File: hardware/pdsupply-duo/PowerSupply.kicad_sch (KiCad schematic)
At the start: 8 parts, among them U5 LTM8026IV#PBF, U6 ACS71240KEXBLT-050U5

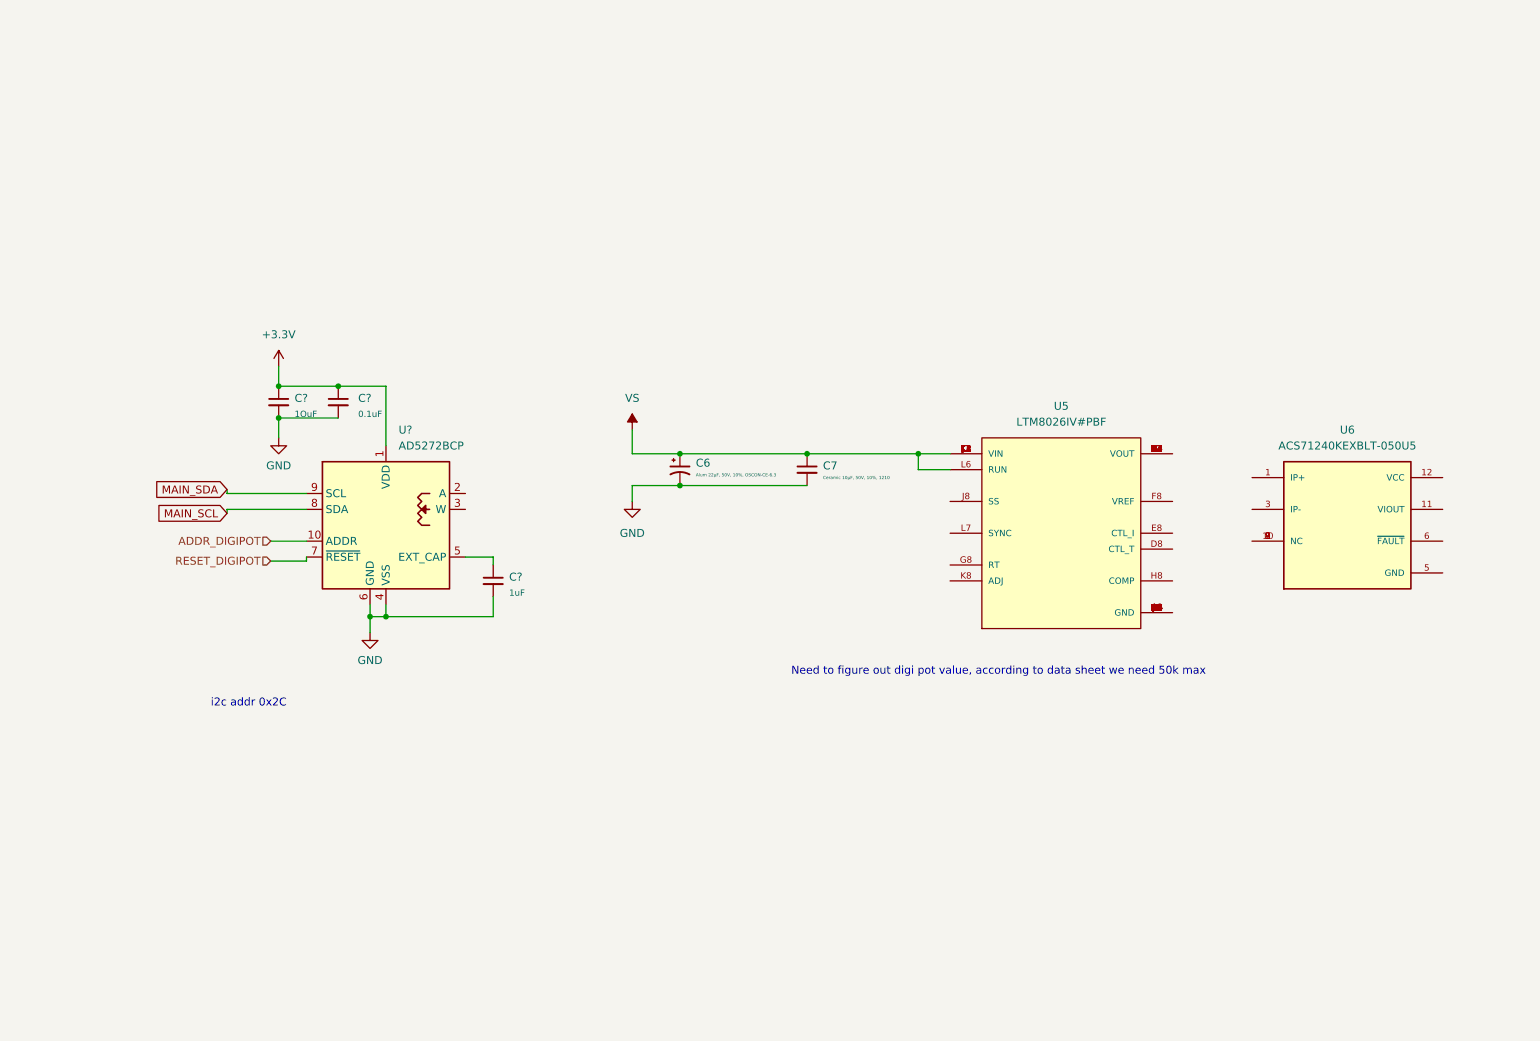
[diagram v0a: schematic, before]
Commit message: SCH 85% done
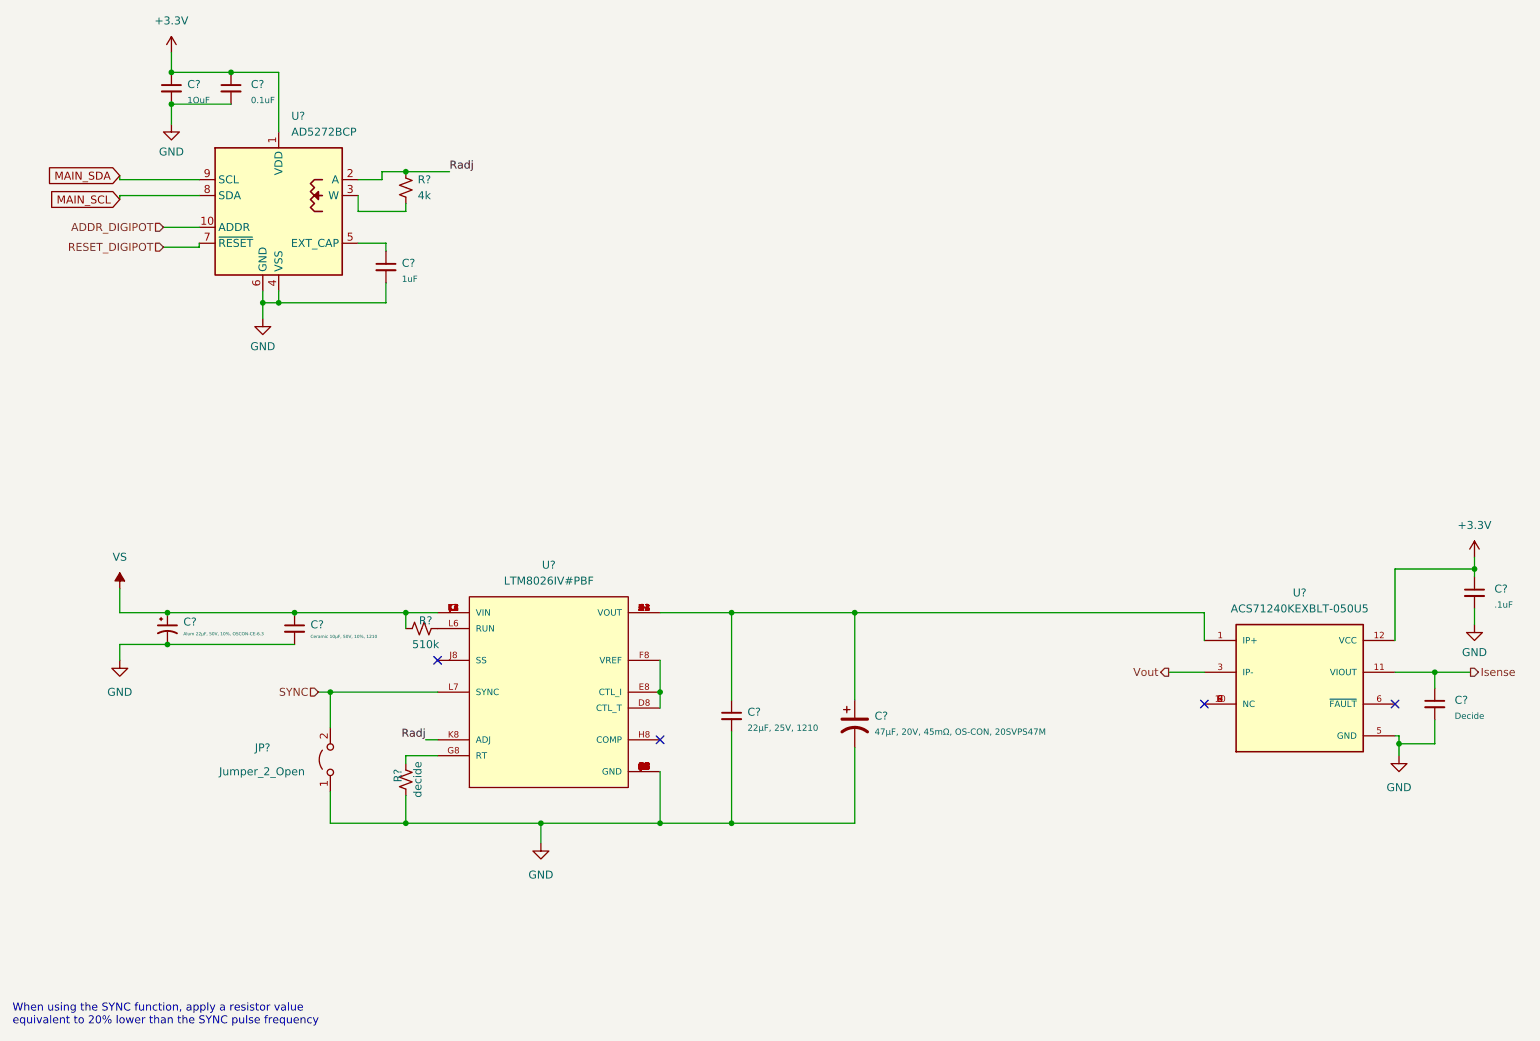
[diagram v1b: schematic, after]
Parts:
- added C?: .1uF, symbol Device:C_Small
- added C?: 22µF, 25V, 1210, symbol Device:C_Small
- added C?: Decide, symbol Device:C_Small
- added C?: 47µF, 20V, 45mΩ, OS-CON, 20SVPS47M, symbol Device:C_Polarized_US
- added JP?: Jumper_2_Open, symbol Jumper:Jumper_2_Open
- added R?: 4k, symbol Device:R_Small_US
- added R?: decide, symbol Device:R_Small_US
- added R?: 510k, symbol Device:R_Small_US
- renumbered C7 to C?, C6 to C?, U6 to U?, U5 to U?
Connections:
- net +3V3: now also U?.12 (VCC), C?.1
- net GND: now also U?.5 (GND), U?.A5 (GND), U?.A6 (GND), U?.A7 (GND), U?.A8 (GND), U?.B5 (GND), U?.B6 (GND), U?.B7 (GND), U?.B8 (GND), U?.C5 (GND), U?.C6 (GND), U?.C7 (GND), U?.C8 (GND), U?.D5 (GND), U?.D6 (GND), U?.D7 (GND), U?.E1 (GND), U?.E2 (GND), U?.E3 (GND), U?.E4 (GND), U?.E5 (GND), U?.E6 (GND), U?.E7 (GND), U?.F1 (GND), U?.F2 (GND), U?.F3 (GND), U?.F4 (GND), U?.F5 (GND), U?.F6 (GND), U?.F7 (GND), U?.G1 (GND), U?.G2 (GND), U?.G3 (GND), U?.G4 (GND), U?.G5 (GND), U?.G6 (GND), U?.G7 (GND), U?.H5 (GND), U?.H6 (GND), U?.H7 (GND), U?.J5 (GND), U?.J6 (GND), U?.J7 (GND), U?.K5 (GND), U?.K6 (GND), U?.K7 (GND), U?.L5 (GND), U?.L8 (GND), C?.2, C?.2, C?.2, C?.2, JP?.1 (A), R?.1
- net VS: now also R?.1; no longer U?.L6 (RUN)
- net at U?.1 (IP+): now also U?.A1 (VOUT), U?.A2 (VOUT), U?.A3 (VOUT), U?.A4 (VOUT), U?.B1 (VOUT), U?.B2 (VOUT), U?.B3 (VOUT), U?.B4 (VOUT), U?.C1 (VOUT), U?.C2 (VOUT), U?.C3 (VOUT), U?.C4 (VOUT), U?.D1 (VOUT), U?.D2 (VOUT), U?.D3 (VOUT), U?.D4 (VOUT), C?.1, C?.1
- net Isense: now reaches U?.11 (VIOUT)
- net Isense: now also C?.1
- net Vout: now reaches U?.3 (IP-)
- net at U?.D8 (CTL_T): now also U?.E8 (CTL_I), U?.F8 (VREF)
- net at U?.G8 (RT): now also R?.2
- net Radj: now reaches U?.K8 (ADJ)
- net Radj: now also U?.2 (A), R?.1
- net SYNC: now reaches U?.L7 (SYNC)
- net SYNC: now also JP?.2 (B)
- net at U?.3 (W): now also R?.2
- new net: R?.2, U?.L6 (RUN)
- no-connect marks 0 -> 4
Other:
- note added: "When using the SYNC function, apply a resistor value equivalent to 20% lower than the SYNC pulse frequency"
- note removed: "Need to figure out digi pot value, according to data sheet we need 50k max"
- note removed: "i2c addr 0x2C"
- moved on the sheet: C?, U?
